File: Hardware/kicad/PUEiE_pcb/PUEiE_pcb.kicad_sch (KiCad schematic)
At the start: 29 parts, among them J1 Screw_Terminal_01x02, J2 USB_C_Receptacle_USB2.0_14P, SW1 SW_DPDT_x2, U1 TPS563240DDC, U2 MAX-M10S-00B, U3 USBLC6-2P6

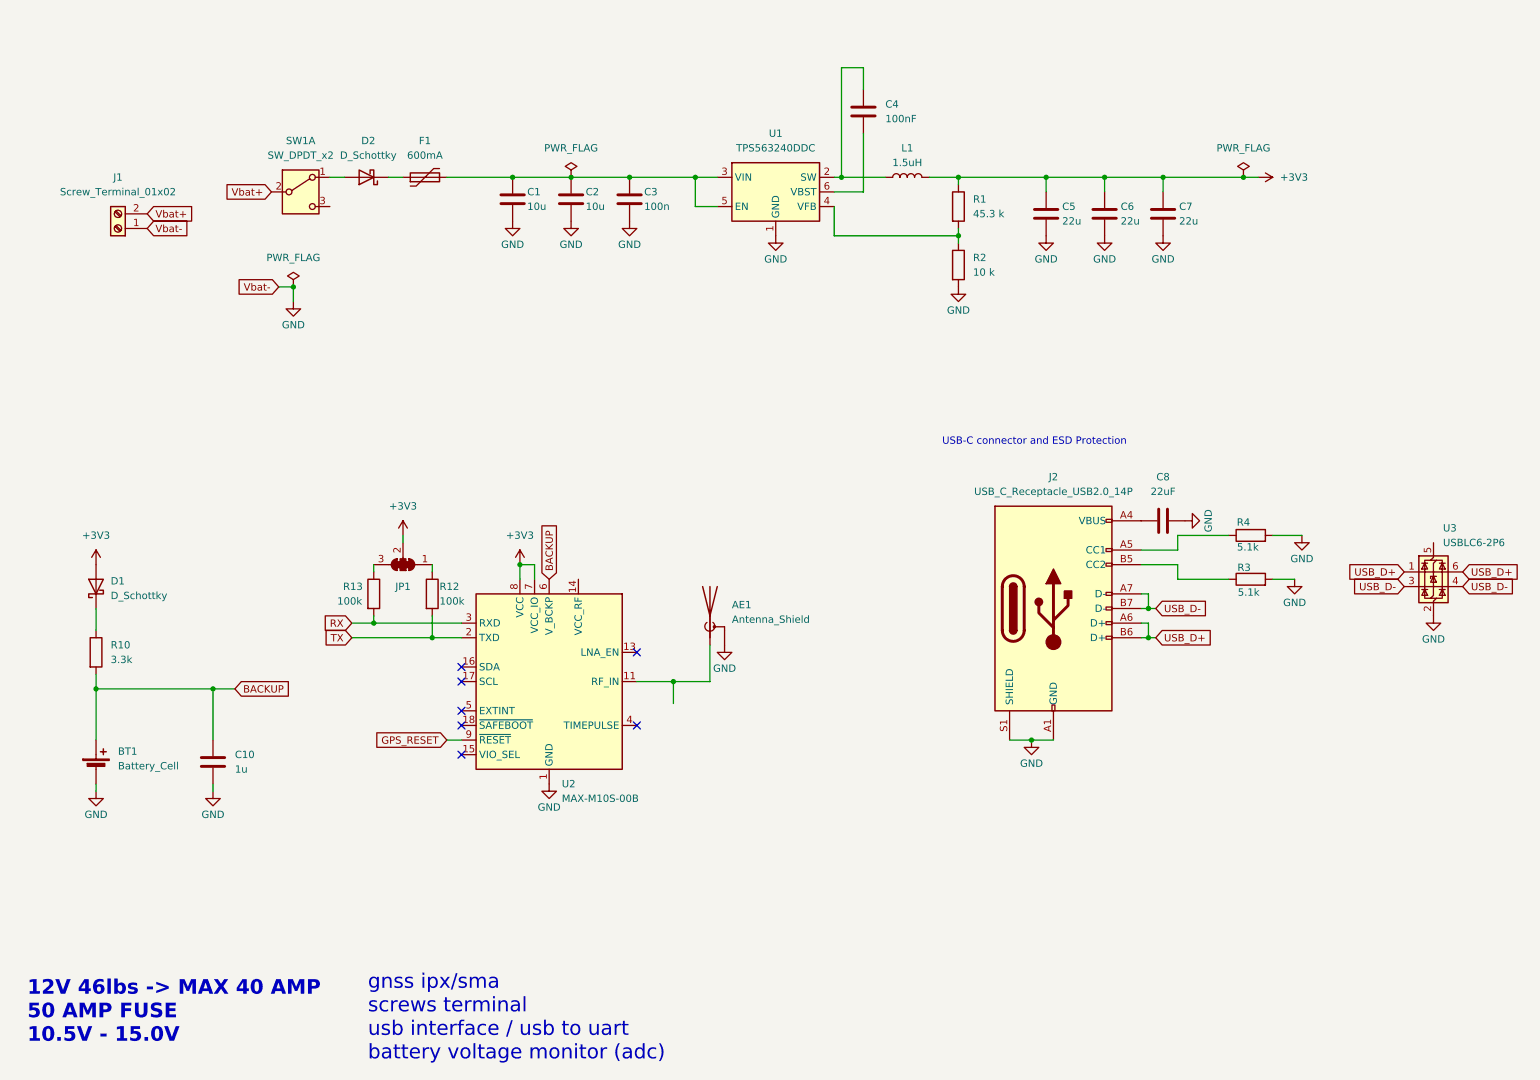
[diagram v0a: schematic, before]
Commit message: cleanup
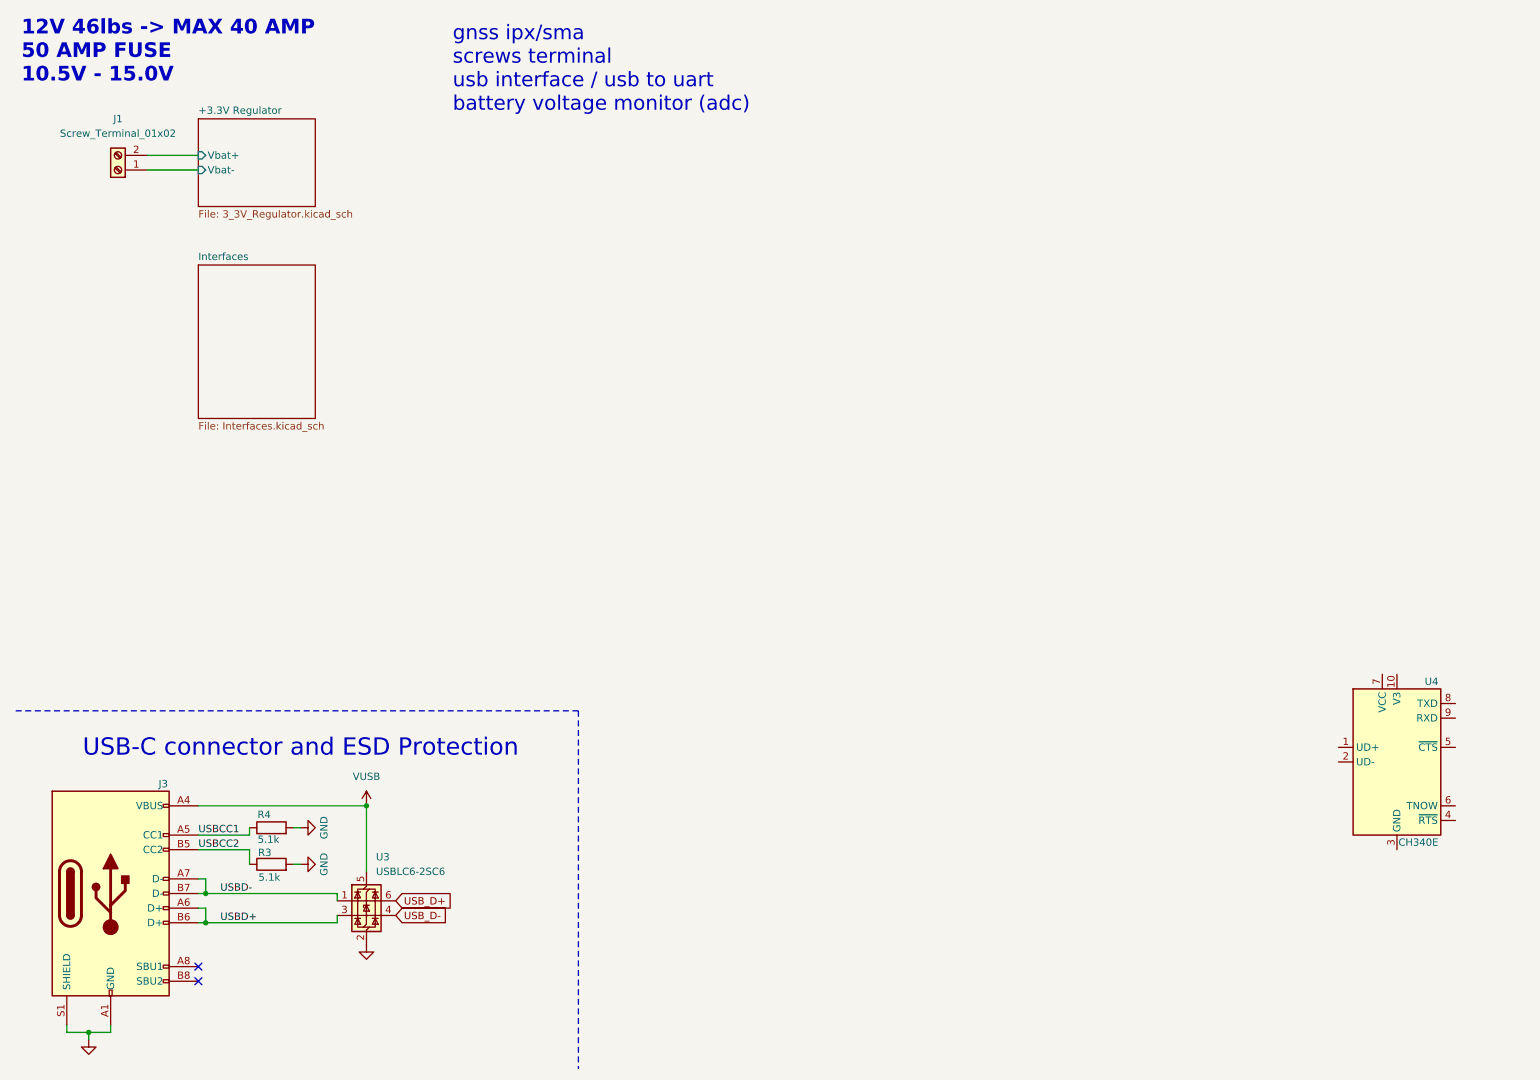
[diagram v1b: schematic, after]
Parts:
- removed AE1: Antenna_Shield, symbol Device:Antenna_Shield
- removed BT1: Battery_Cell, symbol Device:Battery_Cell
- removed C1, C2: 10u, Capacitor_SMD:C_0805_2012Metric, symbol Device:C
- removed C10: 1u, Capacitor_SMD:C_0805_2012Metric, symbol Device:C
- removed C3: 100n, Capacitor_SMD:C_0805_2012Metric, symbol Device:C
- removed C4: 100nF, Capacitor_SMD:C_0603_1608Metric, symbol Device:C
- removed C5, C6, C7: 22u, Capacitor_SMD:C_0603_1608Metric, symbol Device:C
- removed C8: 22uF, symbol Device:C
- removed D1: D_Schottky, Diode_SMD:D_SOD-882, symbol Device:D_Schottky
- removed D2: D_Schottky, symbol Device:D_Schottky
- removed F1: 600mA, symbol Device:Polyfuse
- removed J2: USB_C_Receptacle_USB2.0_14P, symbol Connector:USB_C_Receptacle_USB2.0_14P
- removed JP1: SolderJumper_3_Bridged123, symbol Jumper:SolderJumper_3_Bridged123
- removed L1: 1.5uH, symbol Device:L
- removed R1: 45.3 k, Resistor_SMD:R_0402_1005Metric, symbol Device:R
- removed R10: 3.3k, Resistor_SMD:R_0805_2012Metric, symbol Device:R
- removed R12, R13: 100k, Resistor_SMD:R_0805_2012Metric, symbol Device:R
- removed R2: 10 k, Resistor_SMD:R_0201_0603Metric, symbol Device:R
- removed SW1: SW_DPDT_x2, Button_Switch_THT:SW_E-Switch_EG1224_SPDT_Angled, symbol Switch:SW_DPDT_x2
- removed U1: TPS563240DDC, Package_TO_SOT_SMD:SOT-23-6, symbol Regulator_Switching:TPS563240DDC
- removed U2: MAX-M10S-00B, RF_GPS:ublox_MAX, symbol RF_GPS:MAX-M10S
- removed U3: USBLC6-2P6, Package_TO_SOT_SMD:SOT-666, symbol Power_Protection:USBLC6-2P6
- added J3: USB_C_Receptacle_USB2.0_16P, Connector_USB:USB_C_Receptacle_GCT_USB4105-xx-A_16P_TopMnt_Horizontal, symbol Connector:USB_C_Receptacle_USB2.0_16P
- added U3: USBLC6-2SC6, Package_TO_SOT_SMD:SOT-23-6, symbol Power_Protection:USBLC6-2SC6
- added U4: CH340E, Package_SO:MSOP-10_3x3mm_P0.5mm, symbol Interface_USB:CH340E
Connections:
- net GND: now also J3.A1 (GND), J3.A12 (GND), J3.B1 (GND), J3.B12 (GND), J3.S1 (SHIELD), U3.2 (GND); no longer J1.1 (Pin_1)
- net USB_D+: now also U3.6 (I/O1)
- net USB_D-: now also U3.4 (I/O2)
- net USBCC1: now reaches R4.1
- net USBCC1: now also J3.A5 (CC1)
- net USBCC2: now reaches R3.1
- net USBCC2: now also J3.B5 (CC2)
- net Vbat+ renamed +3.3V Regulator/Vbat+
- new net +3.3V Regulator/Vbat-: J1.1 (Pin_1)
- new net USBD+: J3.A6 (D+), J3.B6 (D+), U3.3 (I/O2)
- new net USBD-: J3.A7 (D-), J3.B7 (D-), U3.1 (I/O1)
- new net VUSB: J3.A4 (VBUS), J3.A9 (VBUS), J3.B4 (VBUS), J3.B9 (VBUS), U3.5 (VBUS)
- no-connect marks 7 -> 2
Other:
- added sheet +3.3V Regulator (3_3V_Regulator.kicad_sch)
- added sheet Interfaces (Interfaces.kicad_sch)
- moved on the sheet: J1, R3, R4
